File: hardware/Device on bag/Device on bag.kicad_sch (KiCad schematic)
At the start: 3 parts, among them U1 STEVAL-MKI215V1, U2 ESP32-DEVKIT-V1, U3 D1_mini_battery_shield

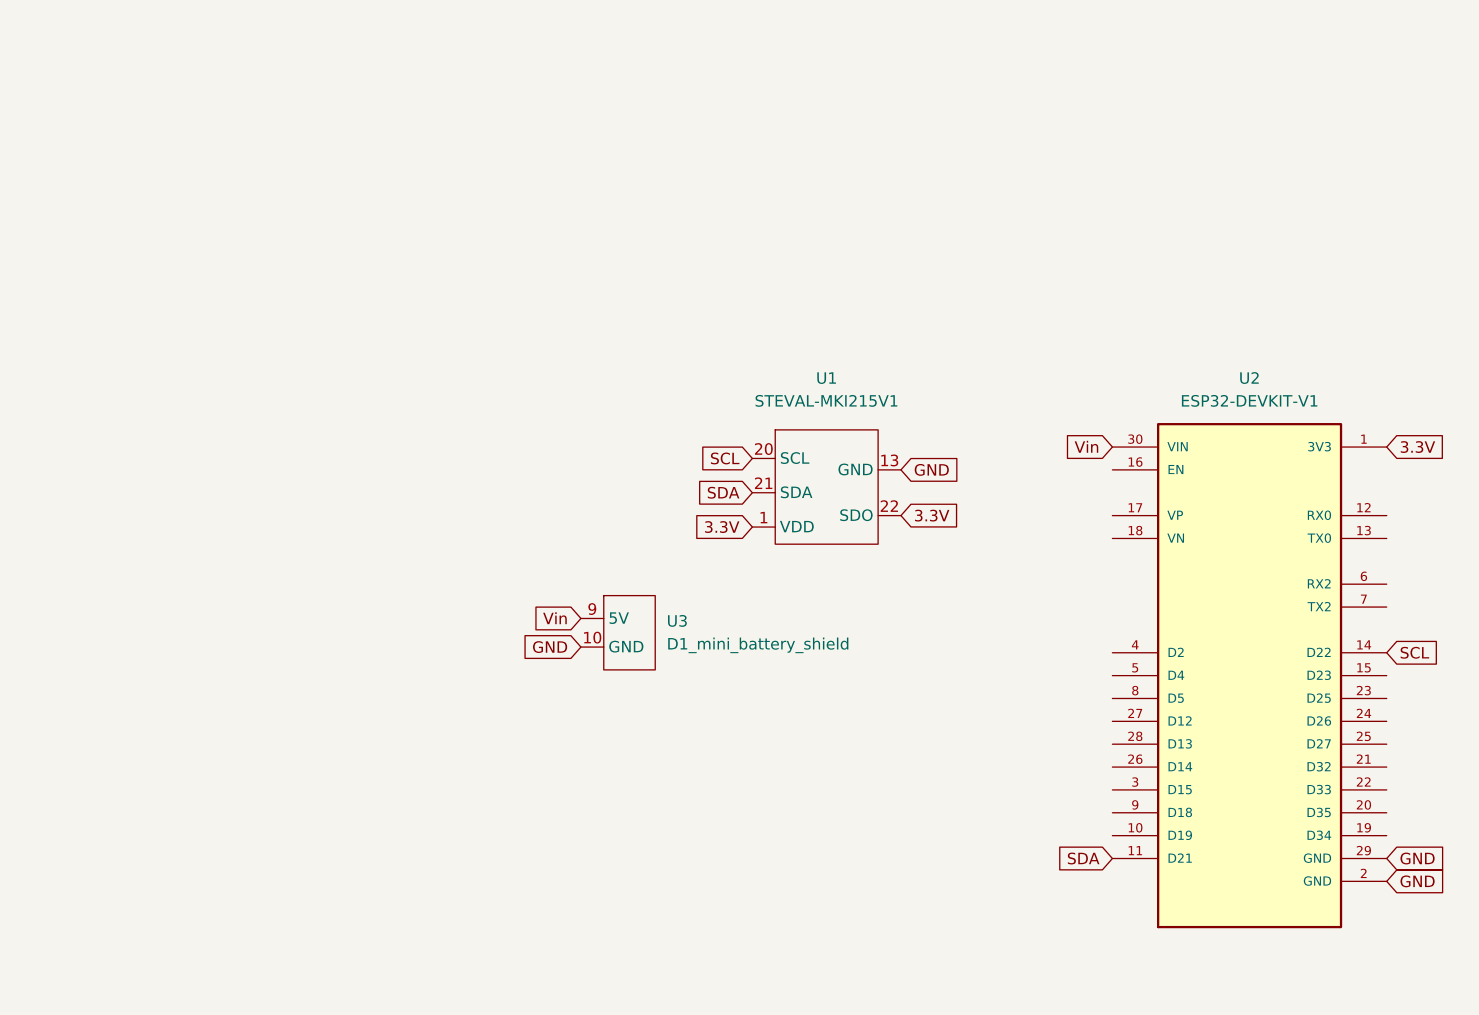
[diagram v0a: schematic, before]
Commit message: update
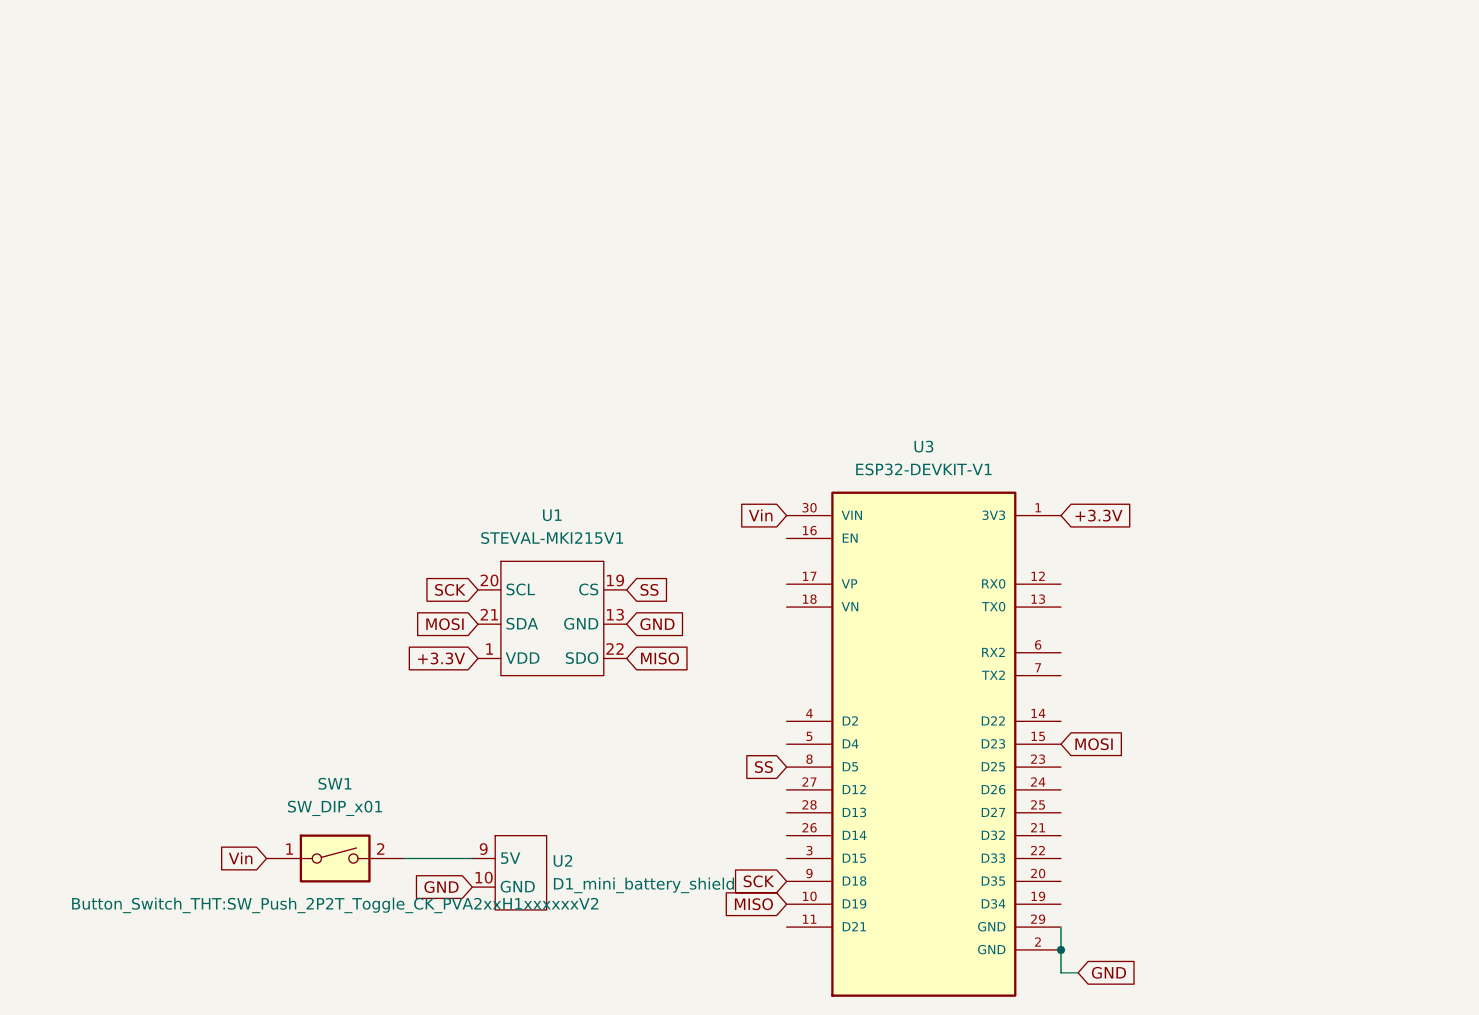
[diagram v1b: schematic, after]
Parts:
- removed U2: ESP32-DEVKIT-V1, MODULE_ESP32_DEVKIT_V1, symbol ESP32-DEVKIT-V1:ESP32-DEVKIT-V1
- removed U3: D1_mini_battery_shield, D1 mini battery shield:D1 mini battery shield, symbol d1 mini battery shield:D1_mini_battery_shield
- added SW1: SW_DIP_x01, Button_Switch_THT:SW_Push_2P2T_Toggle_CK_PVA2xxH1xxxxxxV2, symbol Switch:SW_DIP_x01
- added U2: D1_mini_battery_shield, D1 mini battery shield:D1 mini battery shield, symbol d1 mini battery shield:D1_mini_battery_shield
- added U3: ESP32-DEVKIT-V1, MODULE_ESP32_DEVKIT_V1, symbol ESP32-DEVKIT-V1:ESP32-DEVKIT-V1
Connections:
- net GND: now also U2.10 (GND), U3.2 (GND), U3.29 (GND)
- net Vin: now also SW1.1, U3.30 (VIN)
- net 3.3V renamed +3.3V
- net +3.3V: now also U3.1 (3V3); no longer U1.22 (SDO)
- net SCL renamed SCK
- net SCK: now also U3.9 (D18)
- net SDA renamed MOSI
- net MOSI: now also U3.15 (D23)
- new net: SW1.2, U2.9 (5V)
- new net MISO: U1.22 (SDO), U3.10 (D19)
- new net SS: U1.19 (CS), U3.8 (D5)

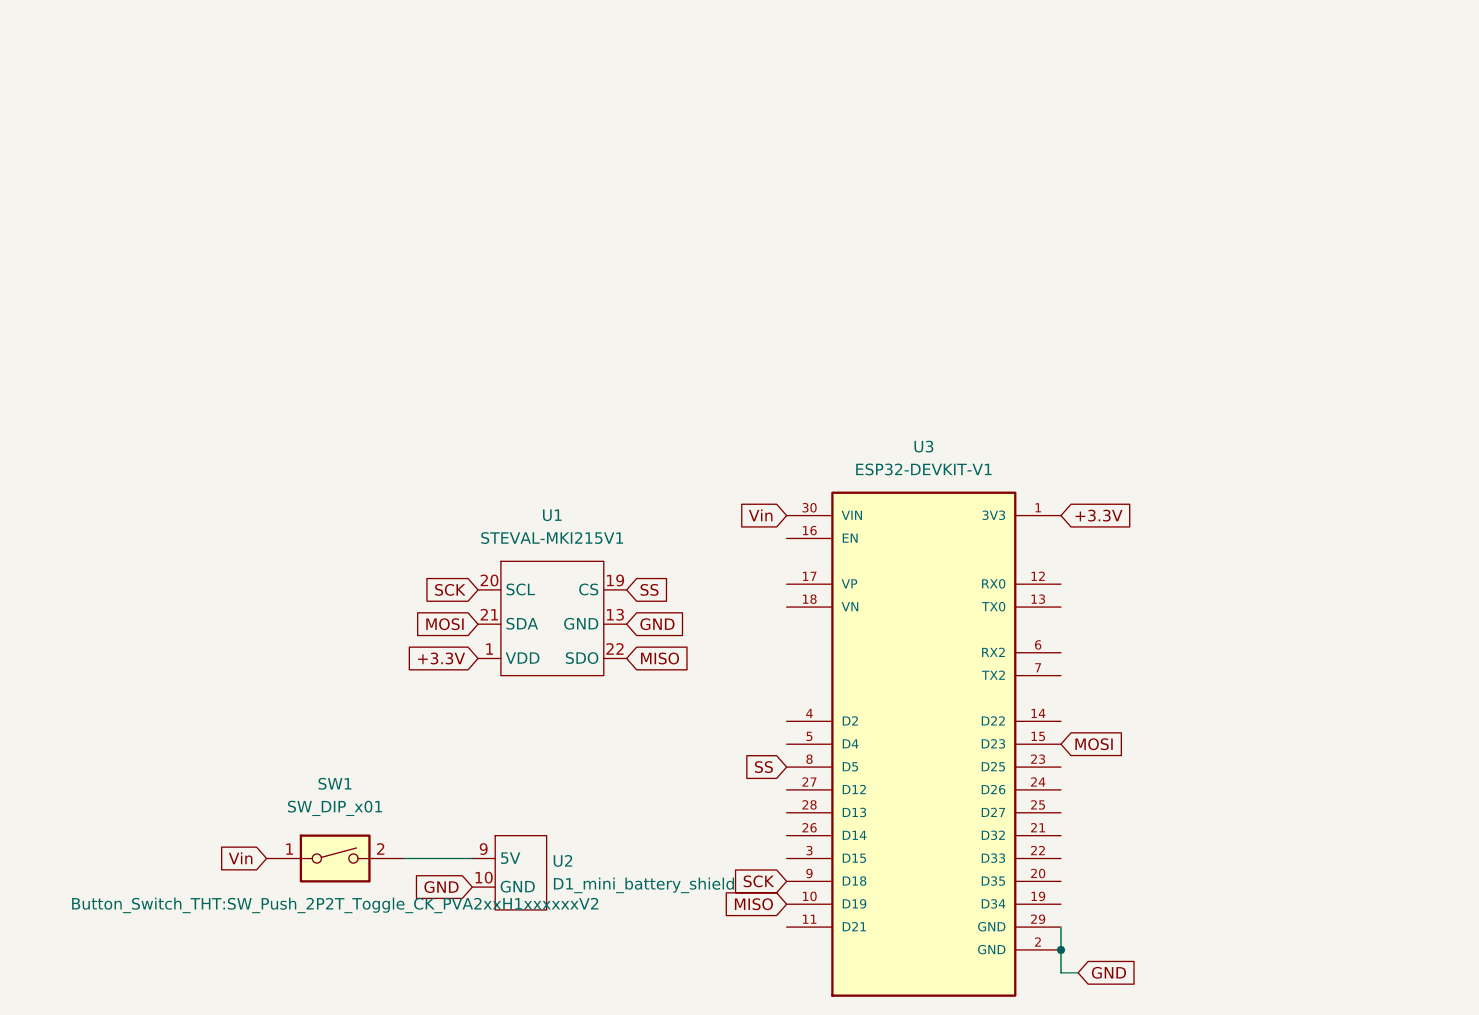
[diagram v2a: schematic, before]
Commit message: init
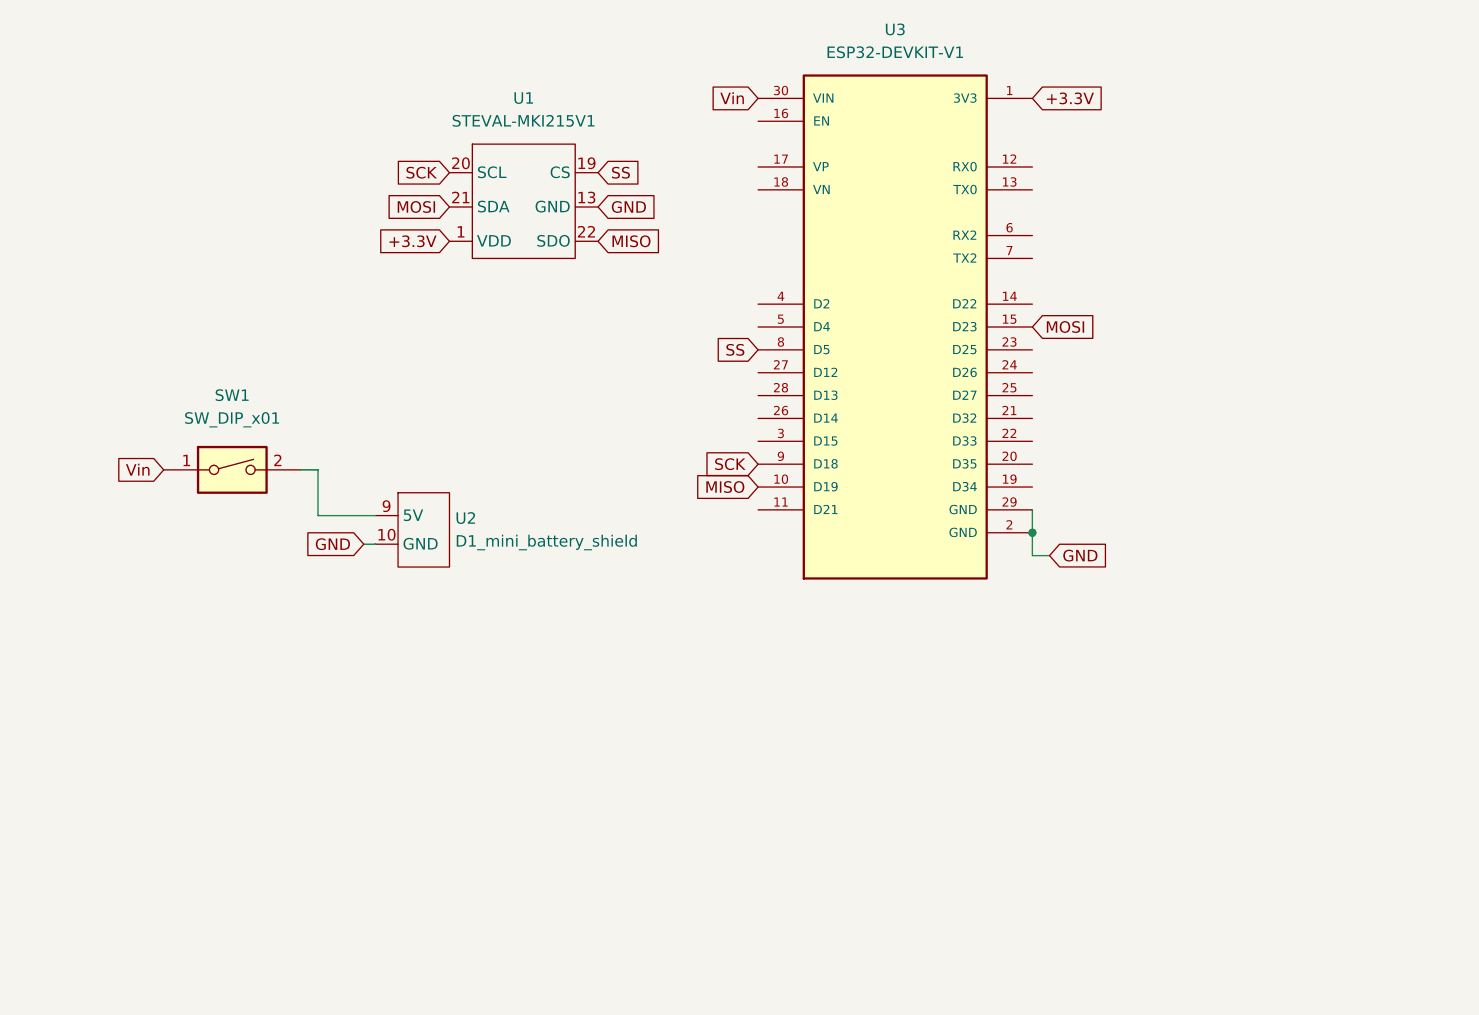
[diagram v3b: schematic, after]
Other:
- title: (none) -> Acceleration/Gyroscope
- moved on the sheet: SW1, U1, U2, U3
